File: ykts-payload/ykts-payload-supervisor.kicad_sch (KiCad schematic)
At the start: 18 parts, among them J8 Conn_02x03_Odd_Even, J9 Conn_01x03_Male, U9 ATmega128A-AU, Y3 8 MHz

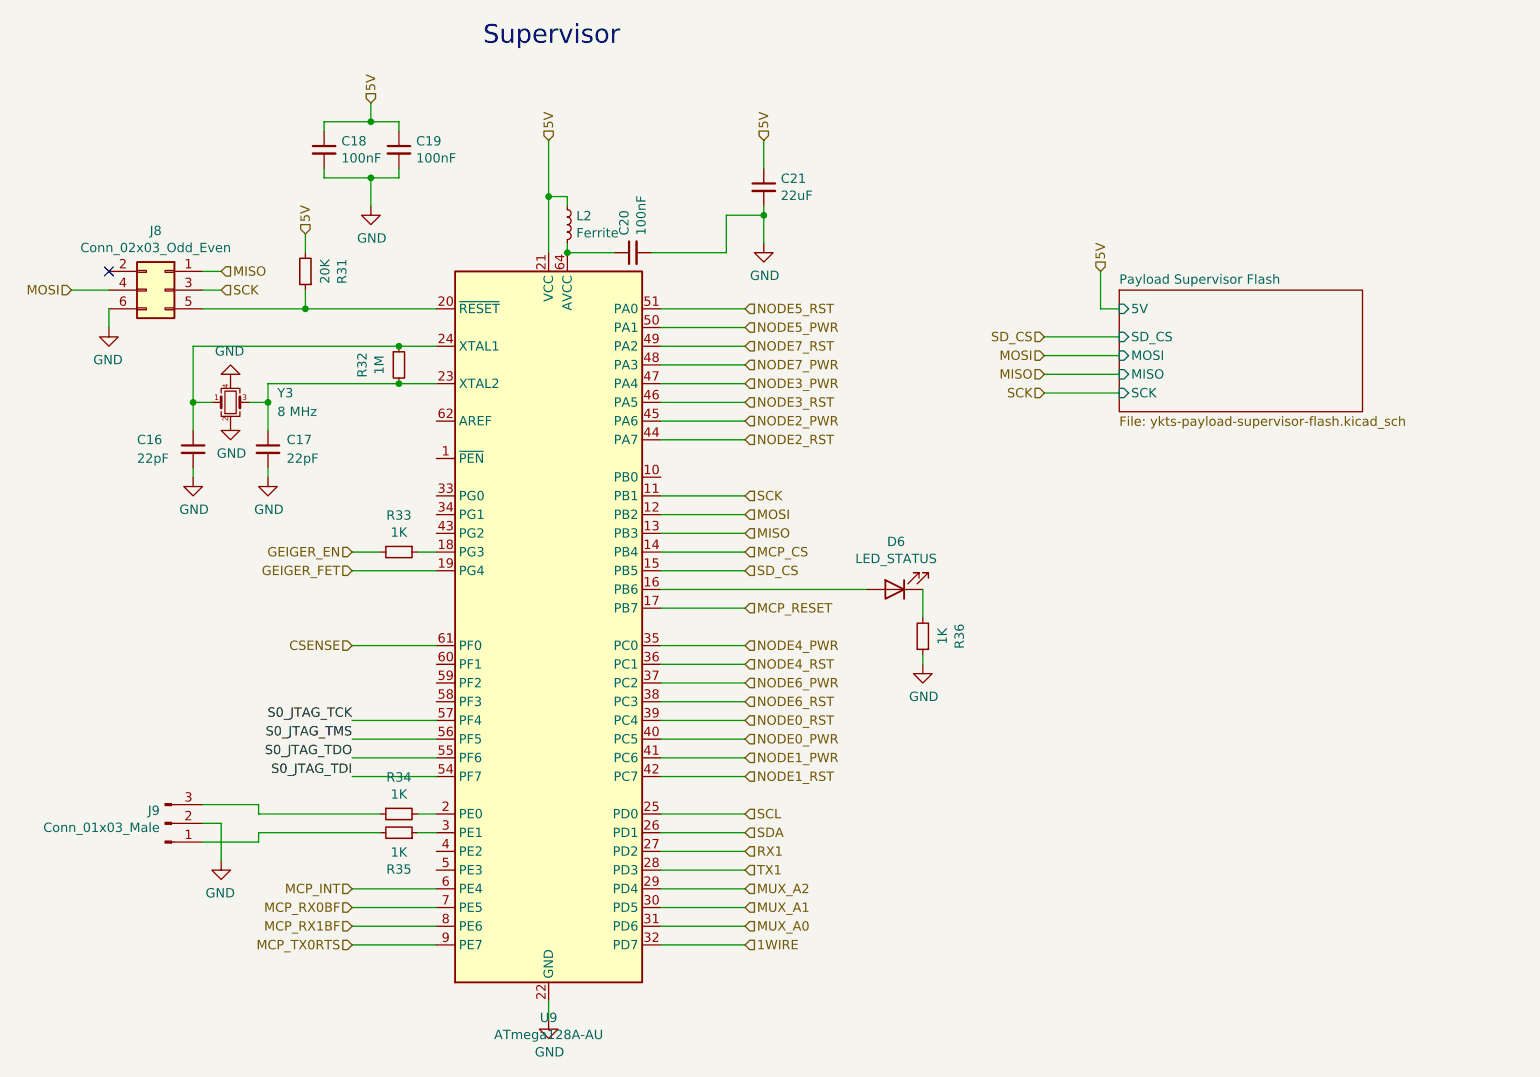
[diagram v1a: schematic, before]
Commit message: Revision A4-Hotfix
Fixed incorrect package for supervisor flash
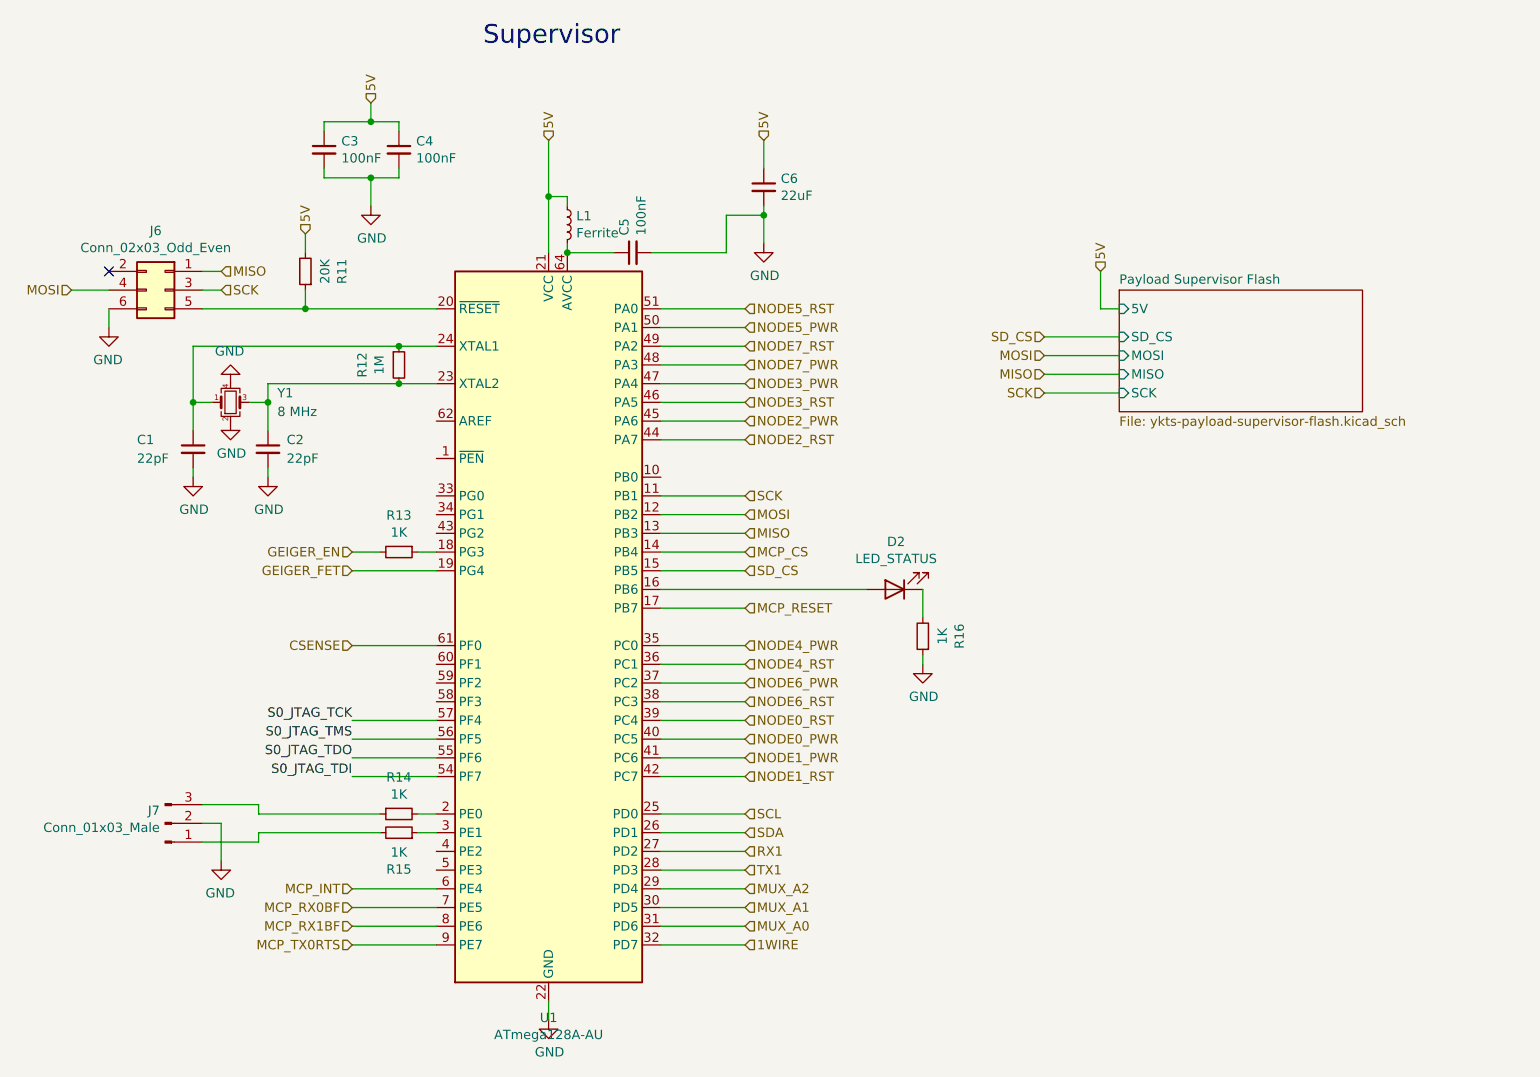
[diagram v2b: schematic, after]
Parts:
- renumbered C16 to C1, C17 to C2, C18 to C3, C19 to C4, C20 to C5, C21 to C6, D6 to D2, J8 to J6, J9 to J7, L2 to L1, R31 to R11, R32 to R12, R33 to R13, R34 to R14, R35 to R15, R36 to R16, U9 to U1, Y3 to Y1
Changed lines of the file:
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@@
   (symbol (lib_id "power:GND") (at 111.76 163.83 0)
     (in_bom yes) (on_board yes)
-    (property "Reference" "#PWR096" (id 0) (at 111.76 170.18 0)
+    (property "Reference" "#PWR067" (id 0) (at 111.76 170.18 0)
       (effects (font (size 1.27 1.27)) hide)
     )
@@
   (symbol (lib_id "Device:C_Small") (at 63.5 86.36 0)
     (in_bom yes) (on_board yes)
-    (property "Reference" "C16" (id 0) (at 55.88 85.09 0)
+    (property "Reference" "C1" (id 0) (at 55.88 85.09 0)
       (effects (font (size 1.27 1.27)) (justify left))
     )
@@
   (symbol (lib_id "Device:C_Small") (at 73.66 86.36 0)
     (in_bom yes) (on_board yes)
-    (property "Reference" "C17" (id 0) (at 76.2 85.09 0)
+    (property "Reference" "C2" (id 0) (at 76.2 85.09 0)
       (effects (font (size 1.27 1.27)) (justify left))
     )
@@
   (symbol (lib_id "power:GND") (at 63.5 90.17 0)
     (in_bom yes) (on_board yes)
-    (property "Reference" "#PWR090" (id 0) (at 63.5 96.52 0)
+    (property "Reference" "#PWR061" (id 0) (at 63.5 96.52 0)
       (effects (font (size 1.27 1.27)) hide)
     )
@@
   (symbol (lib_id "power:GND") (at 73.66 90.17 0)
     (in_bom yes) (on_board yes)
-    (property "Reference" "#PWR094" (id 0) (at 73.66 96.52 0)
+    (property "Reference" "#PWR065" (id 0) (at 73.66 96.52 0)
       (effects (font (size 1.27 1.27)) hide)
     )
@@
   (symbol (lib_id "Device:C_Small") (at 81.28 45.72 0)
     (in_bom yes) (on_board yes)
-    (property "Reference" "C18" (id 0) (at 83.6168 44.5516 0)
+    (property "Reference" "C3" (id 0) (at 83.6168 44.5516 0)
       (effects (font (size 1.27 1.27)) (justify left))
     )
@@
   (symbol (lib_id "Device:C_Small") (at 91.44 45.72 0)
     (in_bom yes) (on_board yes)
-    (property "Reference" "C19" (id 0) (at 93.7768 44.5516 0)
+    (property "Reference" "C4" (id 0) (at 93.7768 44.5516 0)
       (effects (font (size 1.27 1.27)) (justify left))
     )
@@
   (symbol (lib_id "Device:C_Small") (at 123.19 59.69 90)
     (in_bom yes) (on_board yes)
-    (property "Reference" "C20" (id 0) (at 122.0216 57.3532 0)
+    (property "Reference" "C5" (id 0) (at 122.0216 57.3532 0)
       (effects (font (size 1.27 1.27)) (justify left))
     )
@@
   (symbol (lib_id "Device:L_Small") (at 114.3 55.88 0)
     (in_bom yes) (on_board yes)
-    (property "Reference" "L2" (id 0) (at 115.5192 54.7116 0)
+    (property "Reference" "L1" (id 0) (at 115.5192 54.7116 0)
       (effects (font (size 1.27 1.27)) (justify left))
     )
@@
   (symbol (lib_id "power:GND") (at 87.63 53.34 0)
     (in_bom yes) (on_board yes)
-    (property "Reference" "#PWR095" (id 0) (at 87.63 59.69 0)
+    (property "Reference" "#PWR066" (id 0) (at 87.63 59.69 0)
       (effects (font (size 1.27 1.27)) hide)
     )
@@
   (symbol (lib_id "Device:C_Small") (at 140.97 50.8 0)
     (in_bom yes) (on_board yes)
-    (property "Reference" "C21" (id 0) (at 143.2814 49.6316 0)
+    (property "Reference" "C6" (id 0) (at 143.2814 49.6316 0)
       (effects (font (size 1.27 1.27)) (justify left))
     )
@@
   (symbol (lib_id "power:GND") (at 140.97 58.42 0)
     (in_bom yes) (on_board yes)
-    (property "Reference" "#PWR097" (id 0) (at 140.97 64.77 0)
+    (property "Reference" "#PWR068" (id 0) (at 140.97 64.77 0)
       (effects (font (size 1.27 1.27)) hide)
     )
@@
   (symbol (lib_id "Device:Crystal_GND24_Small") (at 68.58 80.01 0)
     (in_bom yes) (on_board yes)
-    (property "Reference" "Y3" (id 0) (at 74.93 78.74 0)
+    (property "Reference" "Y1" (id 0) (at 74.93 78.74 0)
       (effects (font (size 1.27 1.27)) (justify left))
     )
@@
   (symbol (lib_id "power:GND") (at 68.58 77.47 180)
     (in_bom yes) (on_board yes)
-    (property "Reference" "#PWR092" (id 0) (at 68.58 71.12 0)
+    (property "Reference" "#PWR063" (id 0) (at 68.58 71.12 0)
       (effects (font (size 1.27 1.27)) hide)
     )
@@
   (symbol (lib_id "power:GND") (at 68.58 82.55 0)
     (in_bom yes) (on_board yes)
-    (property "Reference" "#PWR093" (id 0) (at 68.58 88.9 0)
+    (property "Reference" "#PWR064" (id 0) (at 68.58 88.9 0)
       (effects (font (size 1.27 1.27)) hide)
     )
@@
   (symbol (lib_id "Device:R_Small") (at 78.74 62.23 180)
     (in_bom yes) (on_board yes)
-    (property "Reference" "R31" (id 0) (at 83.7184 62.23 90))
+    (property "Reference" "R11" (id 0) (at 83.7184 62.23 90))
     (property "Value" "20K" (id 1) (at 81.407 62.23 90))
     (property "Footprint" "Resistor_SMD:R_0402_1005Metric" (id 2) (at 78.74 62.23 0)
@@
   (symbol (lib_id "Device:R_Small") (at 91.44 135.89 90) (mirror x)
     (in_bom yes) (on_board yes)
-    (property "Reference" "R34" (id 0) (at 91.44 130.9116 90))
+    (property "Reference" "R14" (id 0) (at 91.44 130.9116 90))
     (property "Value" "1K" (id 1) (at 91.44 133.223 90))
     (property "Footprint" "Resistor_SMD:R_0402_1005Metric" (id 2) (at 91.44 135.89 0)
@@
   (symbol (lib_id "Device:R_Small") (at 91.44 138.43 270) (mirror x)
     (in_bom yes) (on_board yes)
-    (property "Reference" "R35" (id 0) (at 91.44 143.4084 90))
+    (property "Reference" "R15" (id 0) (at 91.44 143.4084 90))
     (property "Value" "1K" (id 1) (at 91.44 141.097 90))
     (property "Footprint" "Resistor_SMD:R_0402_1005Metric" (id 2) (at 91.44 138.43 0)
@@
   (symbol (lib_id "Device:R_Small") (at 91.44 100.33 270)
     (in_bom yes) (on_board yes)
-    (property "Reference" "R33" (id 0) (at 91.44 95.3516 90))
+    (property "Reference" "R13" (id 0) (at 91.44 95.3516 90))
     (property "Value" "1K" (id 1) (at 91.44 97.663 90))
     (property "Footprint" "Resistor_SMD:R_0402_1005Metric" (id 2) (at 91.44 100.33 0)
@@
   (symbol (lib_id "MCU_Microchip_ATmega:ATmega128A-AU") (at 111.76 110.49 0)
     (in_bom yes) (on_board yes)
-    (property "Reference" "U9" (id 0) (at 111.76 163.5506 0))
+    (property "Reference" "U1" (id 0) (at 111.76 163.5506 0))
     (property "Value" "ATmega128A-AU" (id 1) (at 111.76 165.862 0))
     (property "Footprint" "Package_QFP:TQFP-64_14x14mm_P0.8mm" (id 2) (at 111.76 110.49 0)
@@
   (symbol (lib_id "Device:R_Small") (at 91.44 74.93 0)
     (in_bom yes) (on_board yes)
-    (property "Reference" "R32" (id 0) (at 86.4616 74.93 90))
+    (property "Reference" "R12" (id 0) (at 86.4616 74.93 90))
     (property "Value" "1M" (id 1) (at 88.773 74.93 90))
     (property "Footprint" "Resistor_SMD:R_0402_1005Metric" (id 2) (at 91.44 74.93 0)
@@
   (symbol (lib_id "Connector_Generic:Conn_02x03_Odd_Even") (at 59.69 64.77 0) (mirror y)
     (in_bom yes) (on_board yes)
-    (property "Reference" "J8" (id 0) (at 58.42 56.7182 0))
+    (property "Reference" "J6" (id 0) (at 58.42 56.7182 0))
     (property "Value" "Conn_02x03_Odd_Even" (id 1) (at 58.42 59.0296 0))
     (property "Footprint" "Connector_PinHeader_1.27mm:PinHeader_2x03_P1.27mm_Vertical_SMD" (id 2) (at 59.69 64.77 0)
@@
   (symbol (lib_id "power:GND") (at 52.07 69.85 0) (mirror y)
     (in_bom yes) (on_board yes)
-    (property "Reference" "#PWR089" (id 0) (at 52.07 76.2 0)
+    (property "Reference" "#PWR060" (id 0) (at 52.07 76.2 0)
       (effects (font (size 1.27 1.27)) hide)
     )
@@
   (symbol (lib_id "Connector:Conn_01x03_Male") (at 59.69 137.16 0) (mirror x)
     (in_bom yes) (on_board yes)
-    (property "Reference" "J9" (id 0) (at 58.9788 135.4328 0)
+    (property "Reference" "J7" (id 0) (at 58.9788 135.4328 0)
       (effects (font (size 1.27 1.27)) (justify right))
     )
@@
   (symbol (lib_id "power:GND") (at 67.31 142.24 0) (mirror y)
     (in_bom yes) (on_board yes)
-    (property "Reference" "#PWR091" (id 0) (at 67.31 148.59 0)
+    (property "Reference" "#PWR062" (id 0) (at 67.31 148.59 0)
       (effects (font (size 1.27 1.27)) hide)
     )
@@
   (symbol (lib_id "Device:LED") (at 158.75 105.41 180)
     (in_bom yes) (on_board yes)
-    (property "Reference" "D6" (id 0) (at 158.9278 98.933 0))
+    (property "Reference" "D2" (id 0) (at 158.9278 98.933 0))
     (property "Value" "LED_STATUS" (id 1) (at 158.9278 101.2444 0))
     (property "Footprint" "LED_SMD:LED_0402_1005Metric" (id 2) (at 158.75 105.41 0)
@@
   (symbol (lib_id "power:GND") (at 162.56 115.57 0)
     (in_bom yes) (on_board yes)
-    (property "Reference" "#PWR098" (id 0) (at 162.56 121.92 0)
+    (property "Reference" "#PWR069" (id 0) (at 162.56 121.92 0)
       (effects (font (size 1.27 1.27)) hide)
     )
@@
   (symbol (lib_id "Device:R_Small") (at 162.56 111.76 180)
     (in_bom yes) (on_board yes)
-    (property "Reference" "R36" (id 0) (at 167.5384 111.76 90))
+    (property "Reference" "R16" (id 0) (at 167.5384 111.76 90))
     (property "Value" "1K" (id 1) (at 165.227 111.76 90))
     (property "Footprint" "Resistor_SMD:R_0402_1005Metric" (id 2) (at 162.56 111.76 0)
